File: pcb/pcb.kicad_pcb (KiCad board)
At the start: 2 copper layers, 49 parts, among them J1 GPIO, J2 3.3V Power, J3 3.3V Power, J4 SPI2, J5 SWD, J6 5V Power, J7 5V Power, J8 I2C2, J9 USART1, SW1 SW_Push, SW2 SW_SPDT, SW3 SW_SPDT, U1 STM32F103C8T6, U2 AMS1117-3.3, Y1 8MHz

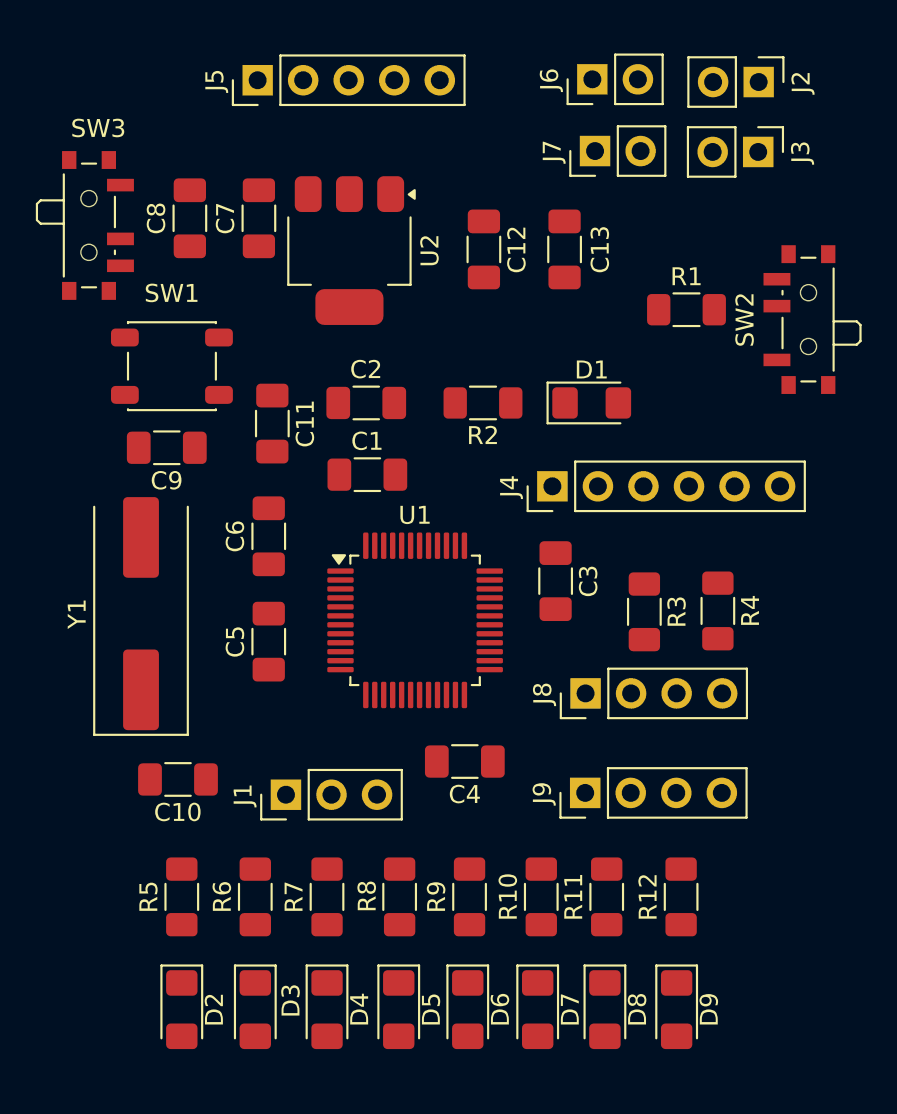
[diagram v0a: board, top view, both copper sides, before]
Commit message: PCB almost done, proctored by Parul
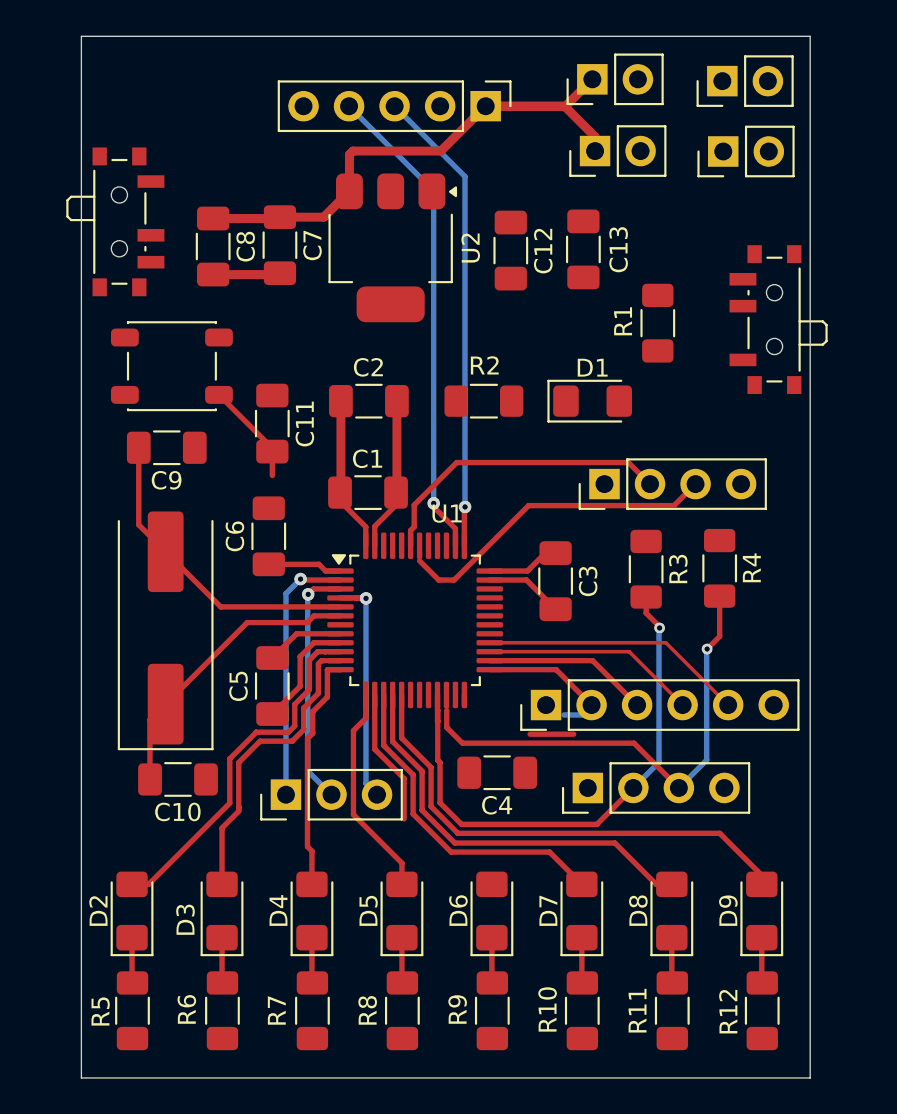
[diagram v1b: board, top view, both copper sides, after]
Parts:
- moved J9 17.3 mm to (100.7, 81.0)
- moved J5 12.8 mm to (94.1, 60.0), turned to -90 degrees
- moved J4 12.2 mm to (97.5, 93.3)
- moved R12 7.80 mm to (109.5, 110.4), turned to -90 degrees
- moved R11 7.33 mm to (104.5, 110.4), turned to -90 degrees
- moved D9 7.27 mm to (109.5, 104.8), turned to 90 degrees
- moved R5 6.92 mm to (74.4, 110.4), turned to -90 degrees
- moved R10 6.75 mm to (99.5, 110.4), turned to -90 degrees
- moved D8 6.65 mm to (104.5, 104.8), turned to 90 degrees
- moved R6 6.61 mm to (79.4, 110.4), turned to -90 degrees
- moved R9 6.48 mm to (94.5, 110.4), turned to -90 degrees
- moved R7 6.40 mm to (84.4, 110.4), turned to -90 degrees
- moved R8 6.35 mm to (89.5, 110.4), turned to -90 degrees
- moved D2 6.16 mm to (74.4, 104.8), turned to 90 degrees
- moved D7 6.03 mm to (99.5, 104.8), turned to 90 degrees
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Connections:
- J4 pad 2: /MISO -> /CS
- J4 pad 3: /MOSI -> /CLK
- J4 pad 4: /CLK -> /MISO
- J4 pad 5: /CS -> /MOSI
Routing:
- net /5V_IN: track 0.00 -> 33.2 mm
- net /SCL: track 0.00 -> 30.4 mm, vias 0 -> 1
- net /LED7: track 0.00 -> 27.4 mm
- net /SWDCLK: track 0.00 -> 27.2 mm, vias 0 -> 1
- net /SDA: track 0.00 -> 26.9 mm, vias 0 -> 1
- net /SWDIO: track 0.00 -> 26.4 mm, vias 0 -> 1
- net +3.3V: track 0.00 -> 23.9 mm
- net /LED6: track 0.00 -> 22.8 mm
- net GND: track 0.00 -> 21.0 mm
- net /LED0: track 0.00 -> 20.1 mm
- net /RX: track 0.00 -> 19.4 mm
- net /LED5: track 0.00 -> 18.4 mm
- net /TX: track 0.00 -> 18.1 mm
- net /HSE_IN: track 0.00 -> 17.4 mm
- net /LED1: track 0.00 -> 16.9 mm
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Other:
- board outline added: 40.7 x 58.1 mm
